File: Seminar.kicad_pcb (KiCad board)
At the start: 2 copper layers, 112.1 x 141.8 mm, 38 parts, among them J1 USB_B_Mini, SW1 SW_Push, SW2 SW_Push, SW3 SPDT, U1 NUCLEO64-F446RE, U2 PCF8574AP, U3 LM2574N-5, U3 TPS61023DRLR, U4 TP4056

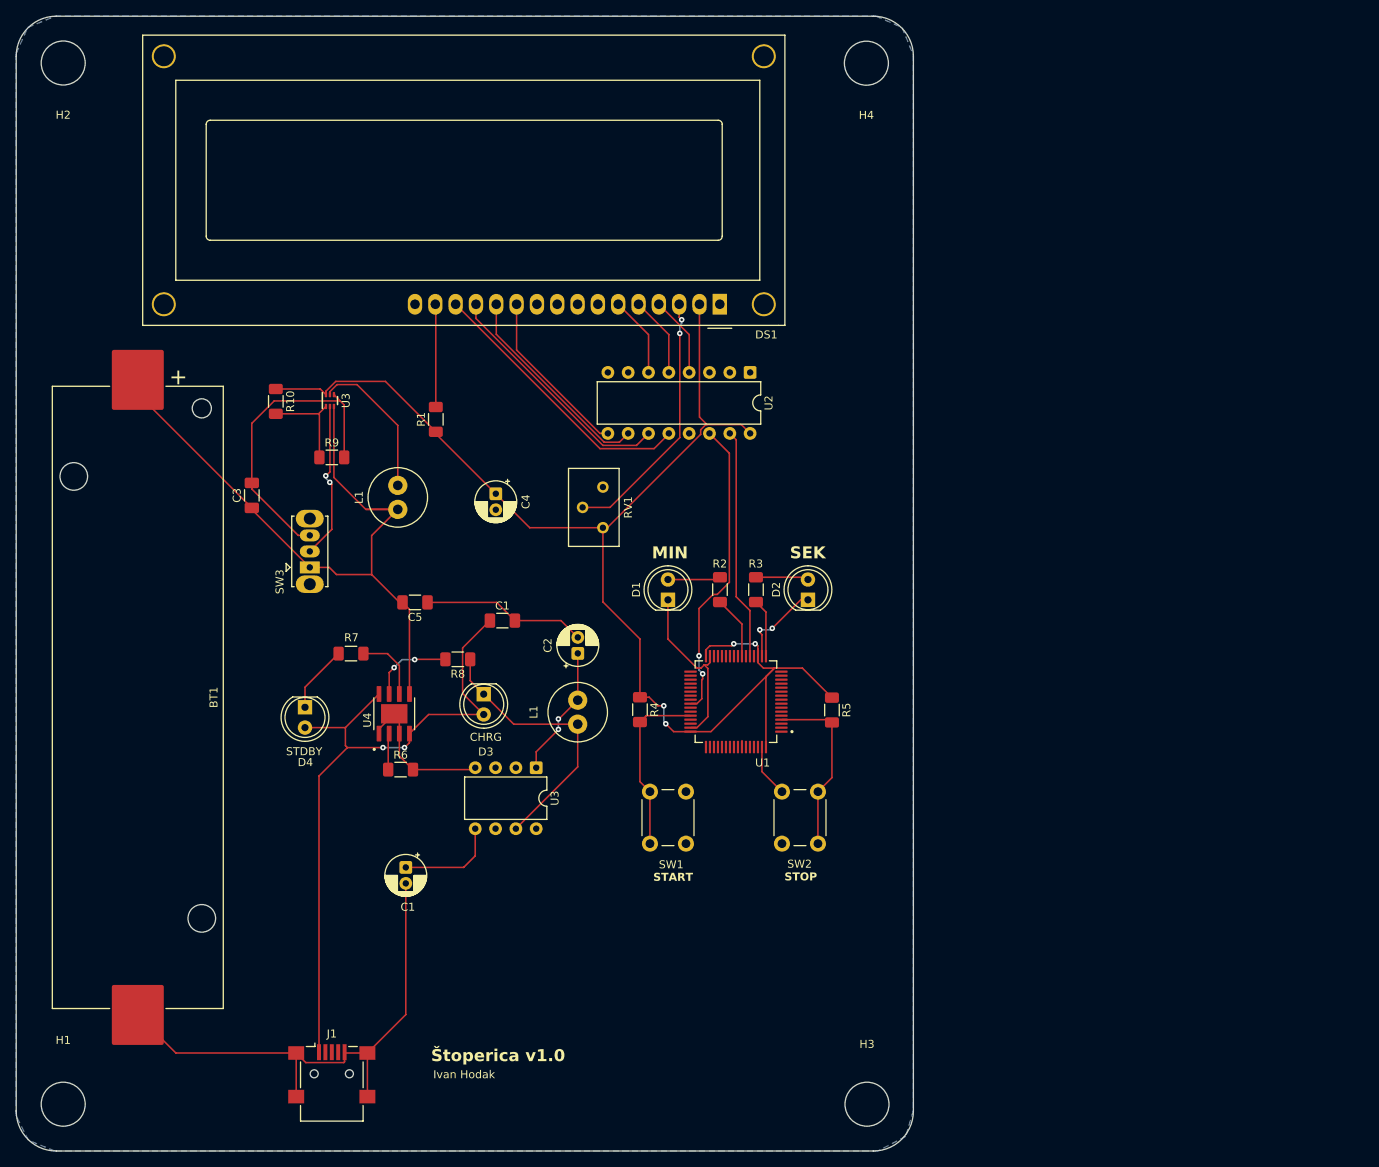
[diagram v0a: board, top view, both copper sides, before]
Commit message: Dorada
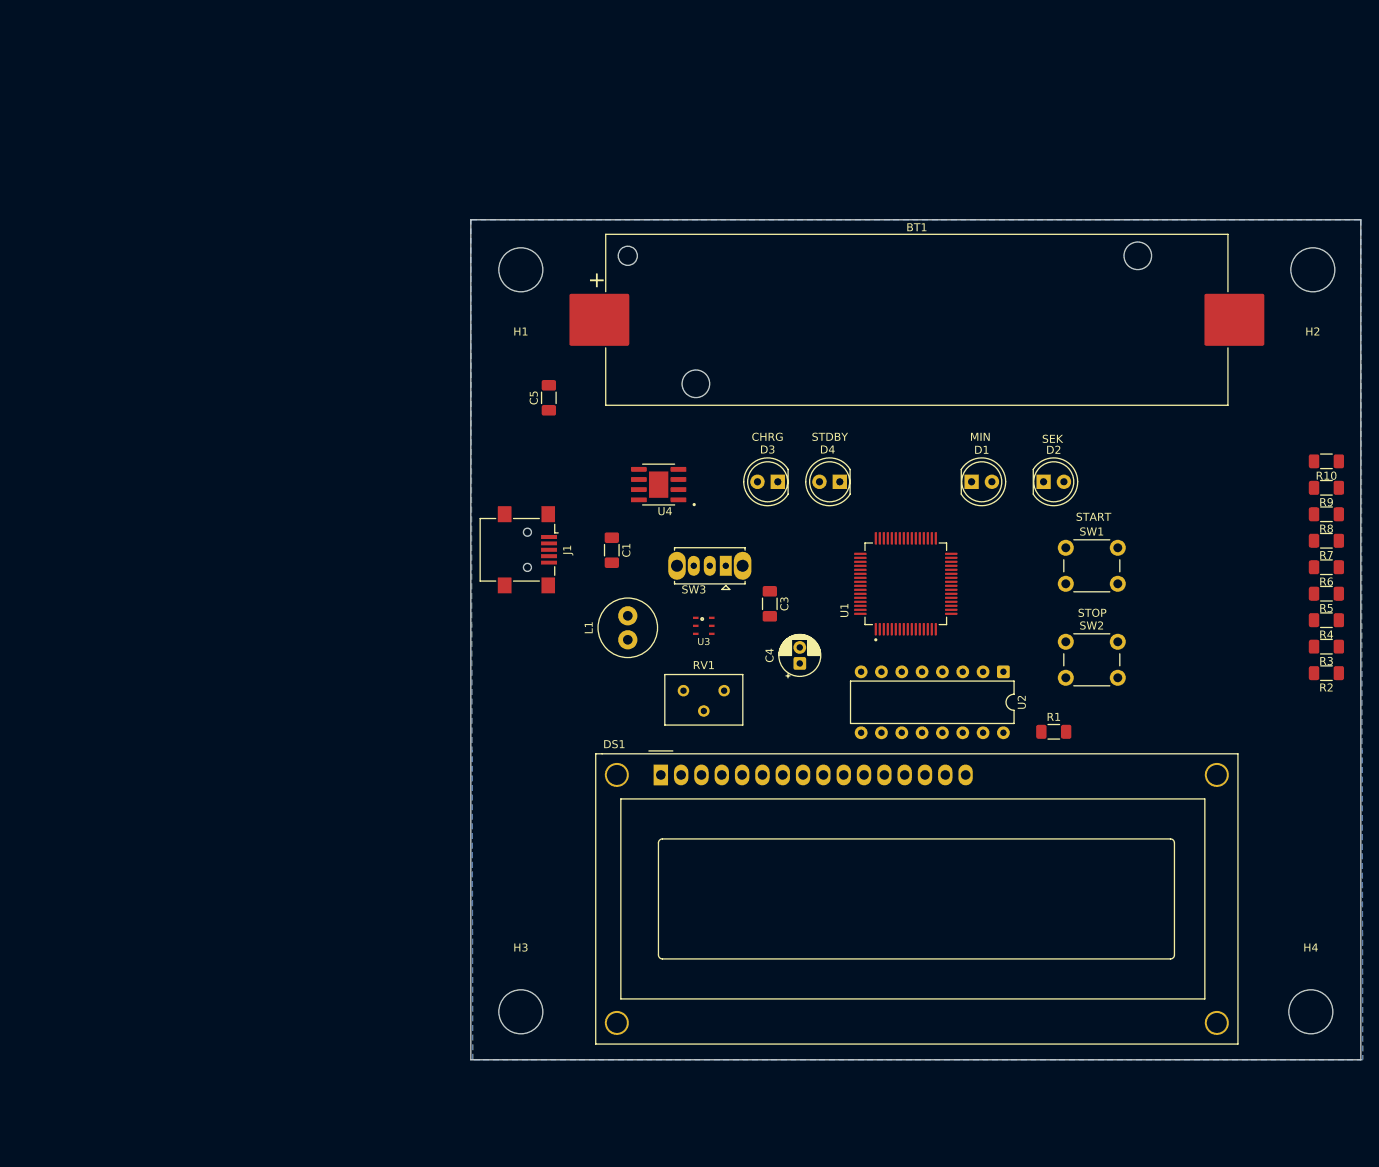
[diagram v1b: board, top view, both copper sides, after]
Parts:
- removed the C1 at (77.5, 124.0)
- removed the C1 at (89.6, 93.1)
- removed C2: 220u, Capacitor_THT:CP_Radial_D5.0mm_P2.00mm
- removed the L1 at (99.0, 106.0)
- removed the L1 at (76.5, 79.2)
- removed the U3 at (93.8, 111.5)
- removed the U3 at (68.0, 65.6)
- added C1: 10u, Capacitor_SMD:C_1206_3216Metric_Pad1.33x1.80mm_HandSolder, F.Cu at (103.2, 84.3)
- added L1: 1u, Inductor_THT:L_Radial_D7.2mm_P3.00mm_Murata_1700, F.Cu at (105.2, 95.5)
- added U3: TPS61023DRLR, footprints:SOT563-ORI, F.Cu at (114.8, 93.5)
- moved H2 158.3 mm to (190.9, 49.2)
- moved R10 131.5 mm to (192.6, 73.2), turned to 180 degrees
- moved H4 130.9 mm to (190.6, 142.0)
- moved R9 124.4 mm to (192.6, 76.5), turned to 180 degrees
- moved R7 122.7 mm to (192.6, 83.1), turned to 180 degrees
- moved H1 119.0 mm to (91.9, 49.2), turned to 0 degrees
- moved R6 118.5 mm to (192.6, 86.4), turned to 180 degrees
- moved R8 110.1 mm to (192.6, 79.8)
- moved BT1 108.2 mm to (141.4, 55.5), turned to 0 degrees
- moved R1 86.6 mm to (158.5, 107.0), turned to 0 degrees
- moved R4 86.5 mm to (192.6, 93.0), turned to 180 degrees
- moved R2 76.5 mm to (192.6, 99.7), turned to 180 degrees
- moved D4 72.5 mm to (131.8, 75.8), turned to 180 degrees
- moved R3 71.7 mm to (192.6, 96.4), turned to 180 degrees
- moved J1 69.9 mm to (92.7, 84.2), turned to -90 degrees
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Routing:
- net GND: track 185.1 -> 0.00 mm, vias 2 -> 0
- net 5V: track 167.3 -> 0.00 mm, vias 4 -> 0
- net +Vin: track 90.5 -> 0.00 mm
- net USB 5V: track 86.8 -> 0.00 mm, vias 2 -> 0
- net SCL: track 38.0 -> 0.00 mm, vias 2 -> 0
- net Net-(DS1-D7): track 34.9 -> 0.00 mm
- net Net-(D3-K): track 34.6 -> 0.00 mm
- net Net-(DS1-VO): track 32.7 -> 0.00 mm, vias 2 -> 0
- net Net-(DS1-D6): track 30.5 -> 0.00 mm
- net SDA: track 28.9 -> 0.00 mm
- net Net-(DS1-D5): track 26.3 -> 0.00 mm
- net START: track 22.4 -> 0.00 mm
- net STOP: track 22.3 -> 0.00 mm
- net Net-(DS1-D4): track 21.4 -> 0.00 mm
- net Net-(SW3-B): track 19.8 -> 0.00 mm, vias 2 -> 0
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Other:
- board size 112.1 x 141.8 mm -> 111.2 x 105 mm
- board text removed: "Ivan Hodak"
- board text removed: "Štoperica v1.0"
